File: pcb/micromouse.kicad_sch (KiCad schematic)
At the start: 25 parts, among them J1 AVR-ISP-6, J2 Conn_01x02, J4 Conn_01x02, J5 Conn_01x04, Q1 Si2319CDS, U1 TSSP77038ETR, U2 TSSP77038ETR, U3 TSSP77038ETR, U4 TSSP77038ETR, U5 TSSP77038ETR, U6 TSSP77038ETR, U7 ATmega328PB-A, U8 MX1508, Y1 Crystal

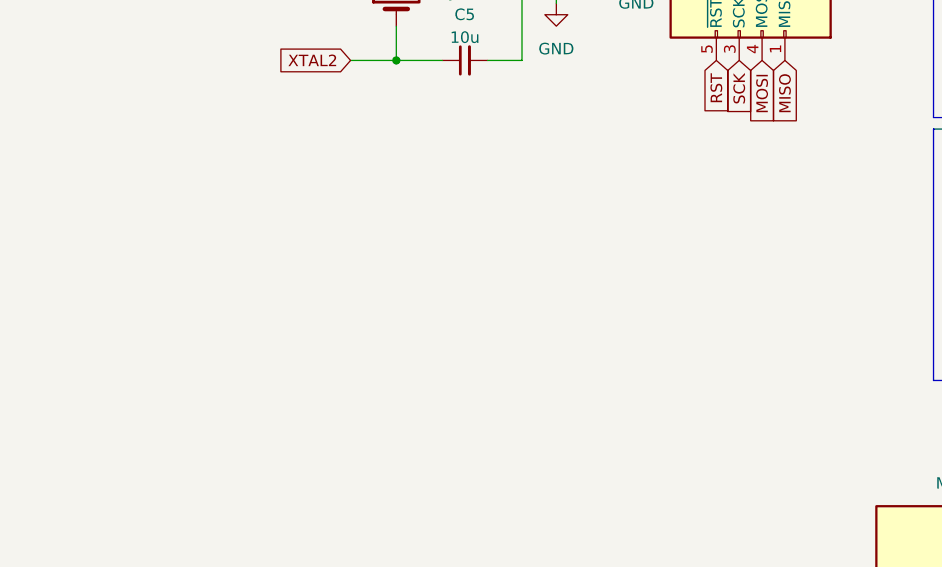
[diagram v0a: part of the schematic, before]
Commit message: update link
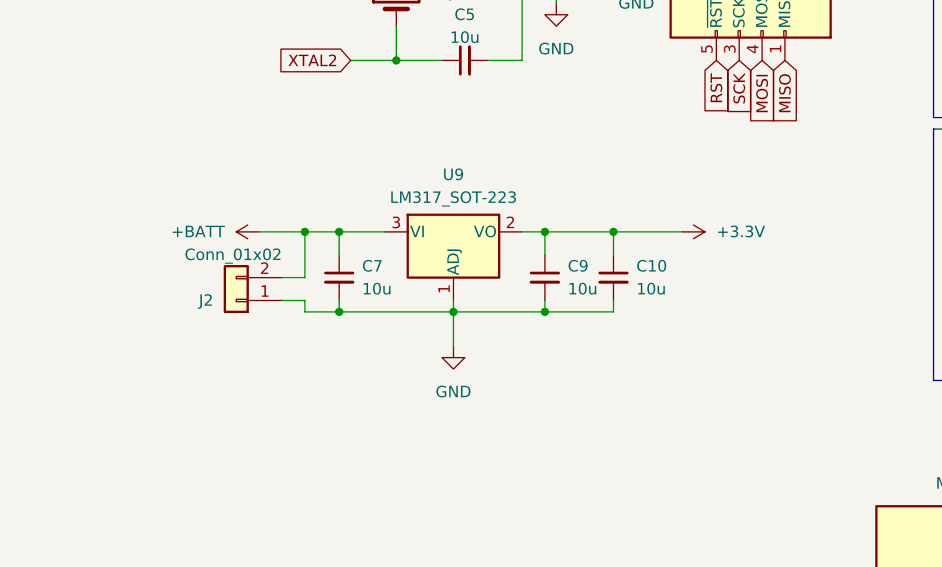
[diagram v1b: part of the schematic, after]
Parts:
- added C10, C7, C9: 10u, Capacitor_SMD:C_0603_1608Metric, symbol Device:C_Small
- added J2: Conn_01x02, Connector_PinSocket_2.54mm:PinSocket_1x02_P2.54mm_Vertical, symbol Connector_Generic:Conn_01x02
- added U9: LM317_SOT-223, Package_TO_SOT_SMD:SOT-223-3_TabPin2, symbol Regulator_Linear:LM317_SOT-223
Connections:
- net +3.3V: now also C10.1, C9.1, U9.2 (VO)
- net +BATT: now also C7.1, J2.2 (Pin_2), U9.3 (VI)
- net GND: now also C10.2, C7.2, C9.2, J2.1 (Pin_1), U9.1 (ADJ)
